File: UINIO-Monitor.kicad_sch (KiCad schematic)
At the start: 49 parts, among them J1 Conn_01x09_Male, J2 Conn_01x09_Male, J3 Conn_01x04_Male, J4 Conn_01x09_Male, P1 LCD_Pad_10Pin, P2 LCD_Pad_12Pin, P3 OLED_Pad_30Pin, P4 LCD_Pad_13Pin, U1 ME6211, U2 ME6211, U3 XC6206PxxxMR, U4 ME6211

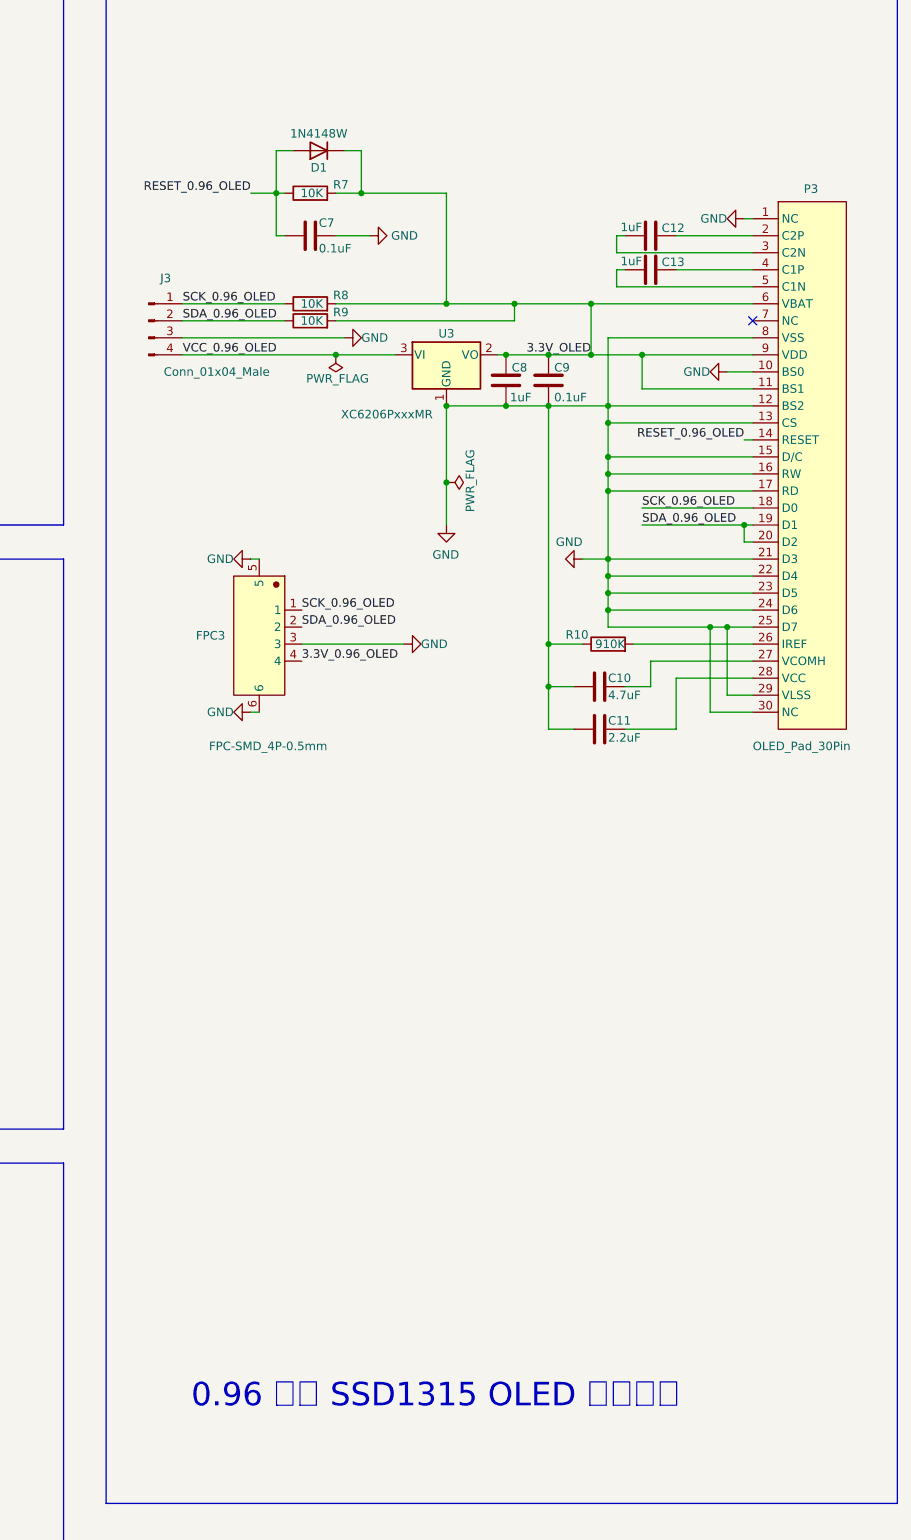
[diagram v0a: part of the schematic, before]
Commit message: Update
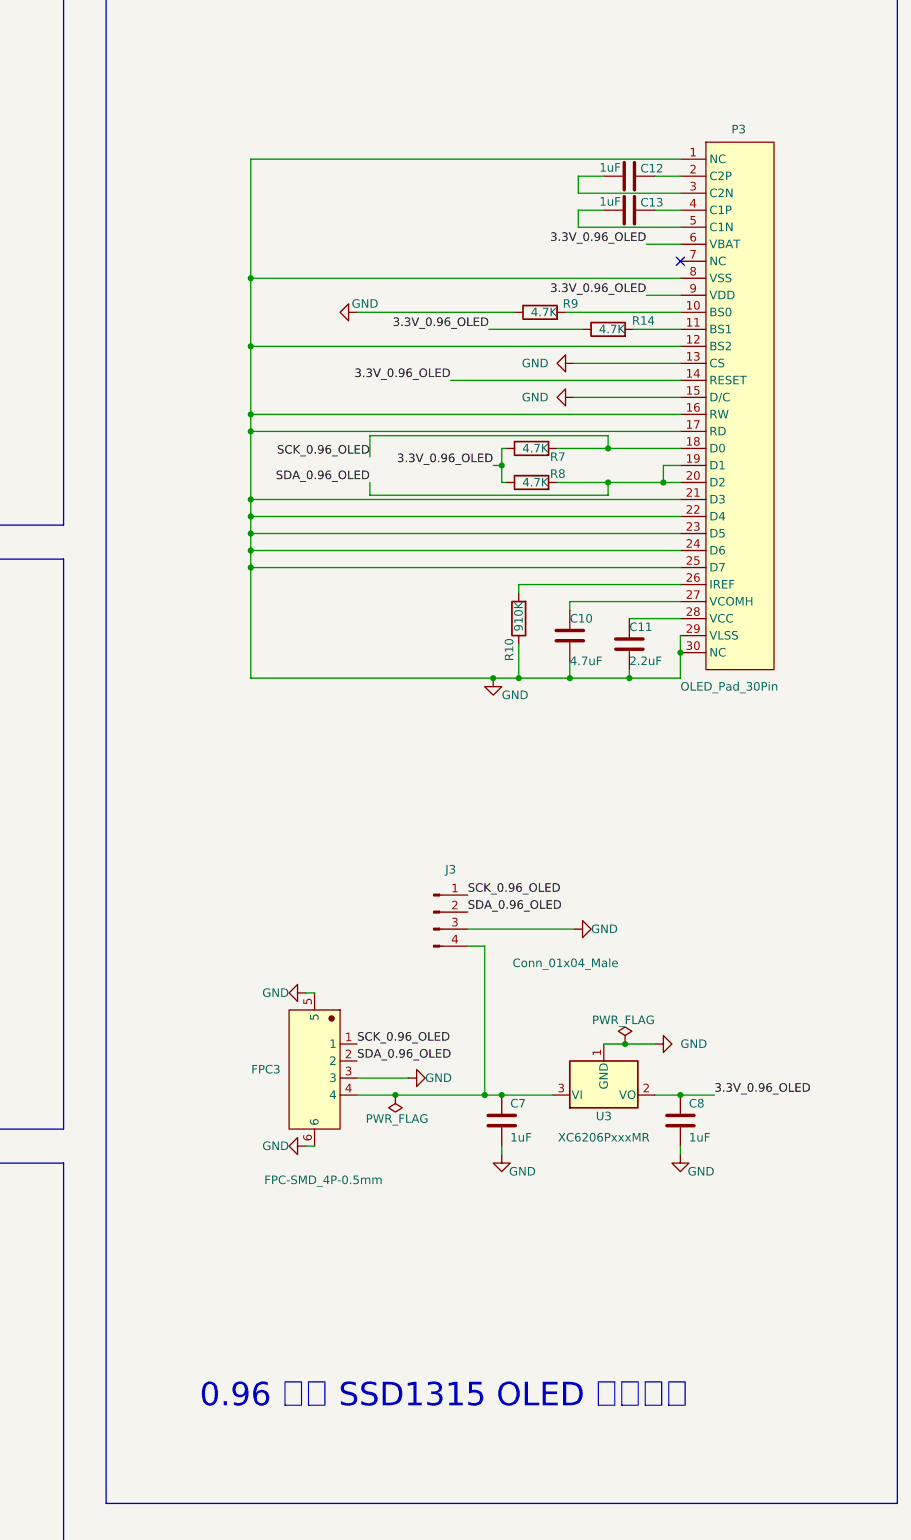
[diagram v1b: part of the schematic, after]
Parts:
- removed C9: 0.1uF, Capacitor_SMD:C_0402_1005Metric, symbol Device:C
- removed D1: 1N4148W, Diode_SMD:D_SOD-123, symbol Diode:1N4148W
- added R14: 4.7K, Resistor_SMD:R_0603_1608Metric, symbol Device:R
- C7: value 0.1uF -> 1uF
- FPC1, FPC2, FPC4: footprint Uinio:FPC-SMD_KH-FG0.5-H2.0-10Pin -> Uinio:FPC-SMD_10P-P0.5
- R7, R8, R9: value 10K -> 4.7K; footprint Resistor_SMD:R_0402_1005Metric -> Resistor_SMD:R_0603_1608Metric
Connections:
- net 3.3V_0.96_OLED: now also C8.1, P3.14 (RESET), P3.6 (VBAT), P3.9 (VDD), R7.1, R8.1, U3.2 (VO), R14.1; no longer FPC3.4
- net GND: now also C7.2, C8.2, R9.1; no longer C7.1, C8.1, P3.10 (BS0)
- net SCK_0.96_OLED: now also R7.2; no longer R8.1
- net SDA_0.96_OLED: now also R8.2; no longer R9.1
- removed net 3.3V_OLED: C8.2, P3.11 (BS1), P3.6 (VBAT), P3.9 (VDD), R7.2, R8.2, R9.2, U3.2 (VO)
- removed net RESET_0.96_OLED: C7.2, P3.14 (RESET), R7.1
- net VCC_0.96_OLED: no longer names the net of J3.4 (Pin_4), U3.3 (VI)
- net VCC_0.96_OLED: now also C7.1, FPC3.4
- new net: P3.10 (BS0), R9.2
- new net: P3.11 (BS1), R14.2
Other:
- moved on the sheet: C10, C11, C12, C13, FPC3, J3, P3, R10, U3
